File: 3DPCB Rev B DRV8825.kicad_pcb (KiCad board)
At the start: 2 copper layers, 100 x 60 mm, 838 parts, among them IC1 DRV8825, IC2 DRV8825, IC3 DRV8825, IC4 DRV8825, IC5 DRV8825, J1 SOLDER_JUMPER_3P, J10 , J11 , J12 , J13 , J14 , J15 , J16 , J2 , J3 , J4 , J5 , J6 , J7 , J8 , J9 , K1 CONN_3, K2 CONN_3, K3 CONN_3, K4 CONN_3, K5 CONN_3, K6 CONN_3, K7 CONN_3, P1 CONN_8, P10 CONN_2, P11 CONN_3X2, P12 CONN_3X2, P13 CONN_4, P2 CONN_2, P3 CONN_2, P4 CONN_2, P5 CONN_4, P6 CONN_4, P7 CONN_4, P8 CONN_2, P9 CONN_4, U1 CONN_4_LERCHE, U10 MICRO-SD, U11 TC4427, U12 MCP4728, U13 CONN_4_LERCHE, U15 SPST_MOMENTARY, U16 CONN_4_LERCHE, U17 TC4427, U2 SPST_MOMENTARY, U20 TPS6213X, U21 CONN_4_LERCHE, U22 CONN_4_LERCHE, U23 MCP4728, U24 MOS_NFET, U25 CONN_4_LERCHE, U3 BSS84, U4 CONN_4_LERCHE, U5 MOS_NFET, U6 LPC1768_TQFP100, U7 MOS_NFET, U8 MOS_NFET, U9 CRYSTAL_SMALL

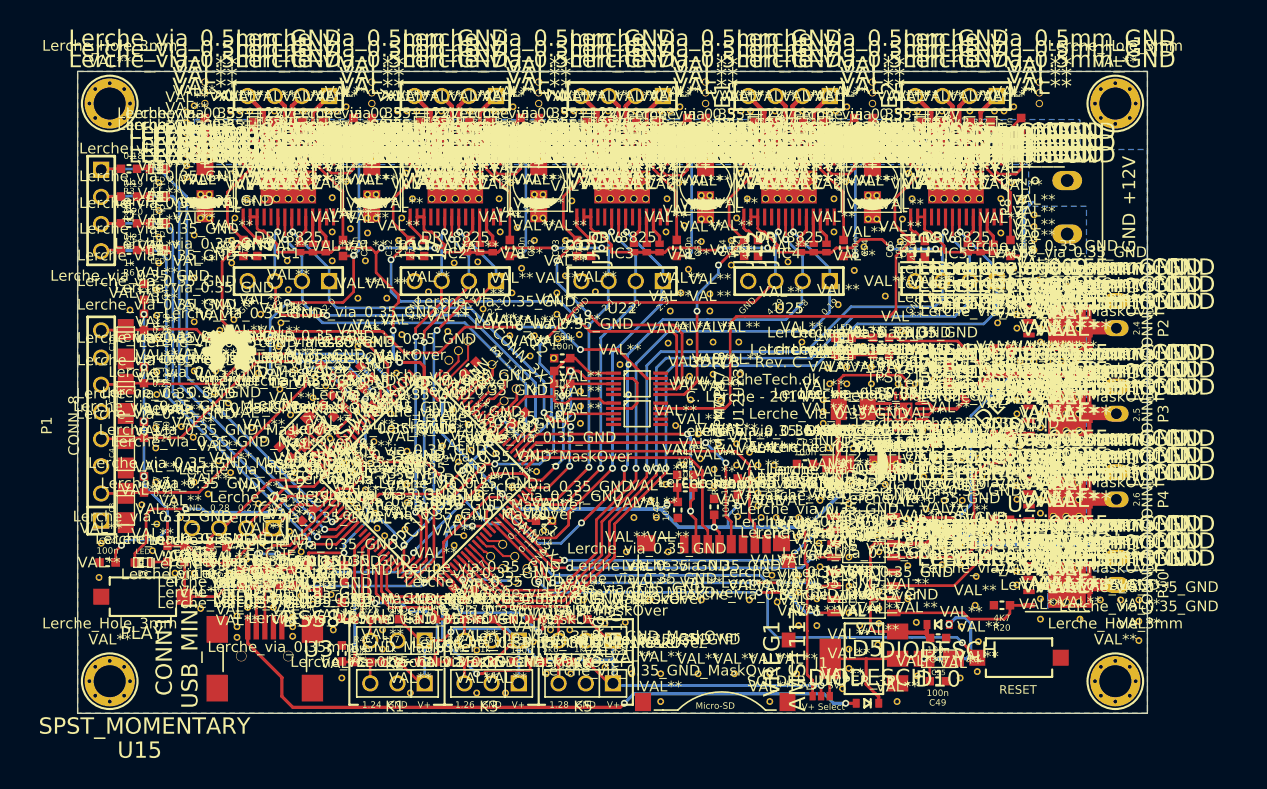
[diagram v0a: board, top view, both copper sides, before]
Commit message: Added LercheTech library
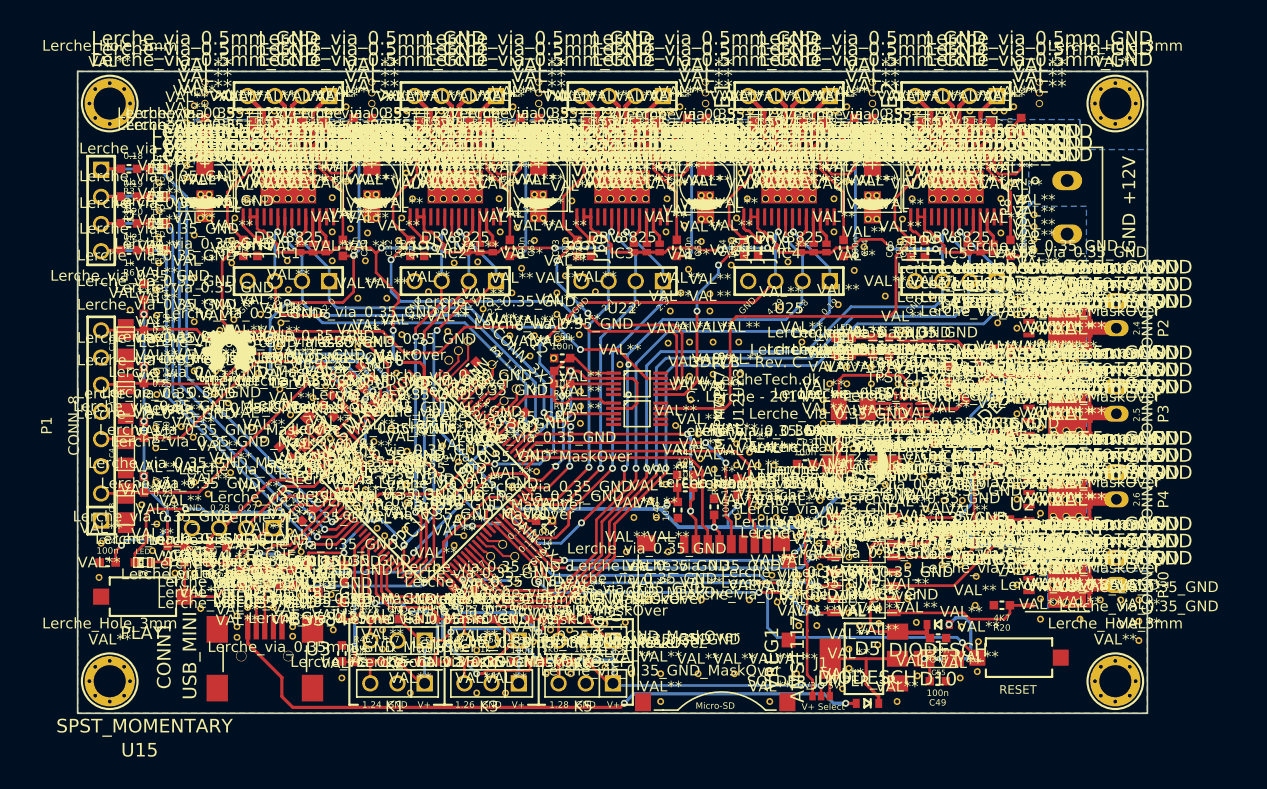
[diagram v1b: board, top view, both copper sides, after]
